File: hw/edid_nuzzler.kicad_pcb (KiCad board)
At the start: 2 copper layers, 49 x 32 mm, 49 parts, among them J1 HDMI_A, J2 HDMI_A, J4 USB_C_Receptacle_USB2.0_16P, J5 Prog, Q1 BSS84AK, SW1 SW_Push, U1 74LVC1G3157, U2 74LVC1G3157, U3 CH340N, U4 CH32V003AxMx, U5 74LVC1G3157, U6 ZD24C16A-STGMT

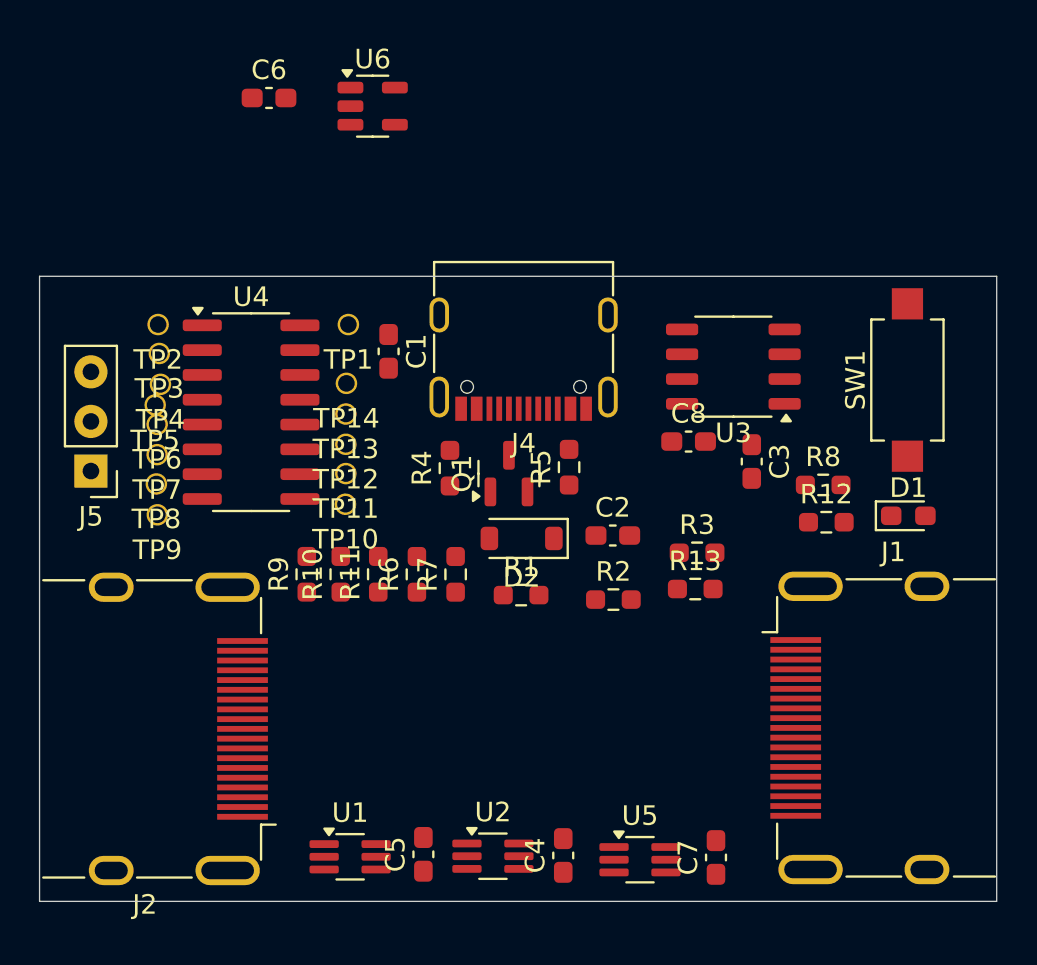
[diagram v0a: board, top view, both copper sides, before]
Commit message: Corase layout
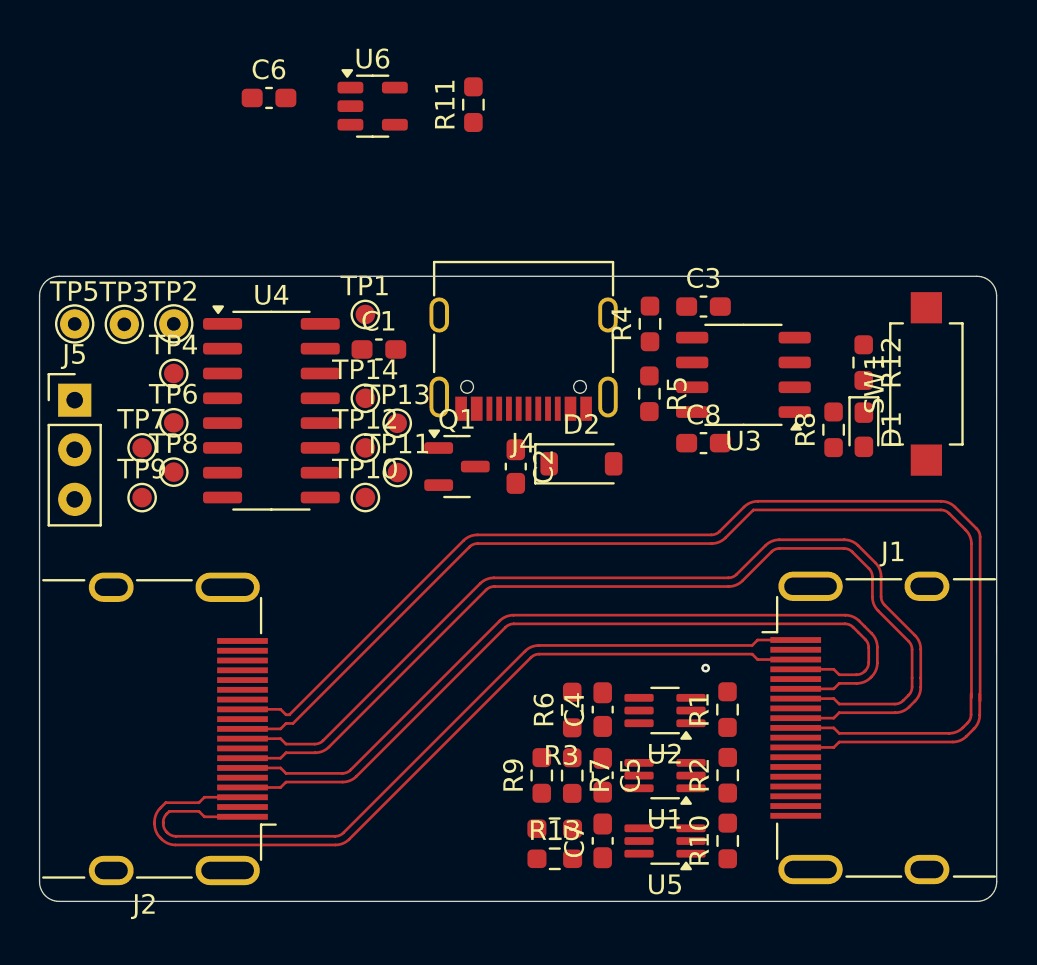
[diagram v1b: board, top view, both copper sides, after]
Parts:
- TP1, TP10, TP11, TP12, TP13, TP14, TP4, TP6, TP7, TP8, TP9: value ~ -> pad; footprint nuzzler:Pin_tight -> TestPoint:TestPoint_Pad_D1.0mm
- TP2, TP3, TP5: footprint nuzzler:Pin_tight -> TestPoint:TestPoint_THTPad_D1.5mm_Drill0.7mm
- moved R11 24.5 mm to (183.6, 53.3)
- moved R10 24.1 mm to (196.6, 91.0)
- moved U1 16.6 mm to (193.4, 87.7), turned to 180 degrees
- moved R3 15.9 mm to (187.8, 90.4)
- moved R9 15.8 mm to (187.1, 87.7)
- moved R13 15.6 mm to (187.8, 91.9)
- moved R4 12.6 mm to (192.7, 64.5)
- moved R1 12.1 mm to (196.6, 84.3), turned to 90 degrees
- moved R7 11.9 mm to (188.7, 87.7), turned to -90 degrees
- moved U2 11.5 mm to (193.4, 84.3), turned to 180 degrees
- moved R2 10.7 mm to (196.6, 87.6), turned to 90 degrees
- moved R6 10.6 mm to (188.7, 84.3)
- moved C5 10.0 mm to (190.2, 87.6), turned to -90 degrees
- moved R12 8.39 mm to (203.6, 66.5), turned to -90 degrees
- moved C3 8.31 mm to (195.4, 63.6), turned to 0 degrees
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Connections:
- net Net-(J1-CK+) renamed /CK+
- net Net-(J1-CK-) renamed /CK-
- net Net-(J1-D0+) renamed /D0+
- net Net-(J1-D0-) renamed /D0-
- net Net-(J1-D1+) renamed /D1+
- net Net-(J1-D1-) renamed /D1-
- net Net-(J1-D2+) renamed /D2+
- net Net-(J1-D2-) renamed /D2-
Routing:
- net /CK-: track 0.00 -> 62.8 mm
- net /CK+: track 0.00 -> 61.2 mm
- net /D0-: track 0.00 -> 51.6 mm
- net /D0+: track 0.00 -> 50.2 mm
- net /D2-: track 0.00 -> 42.8 mm
- net /D1-: track 0.00 -> 42.4 mm
- net /D2+: track 0.00 -> 41.4 mm
- net /D1+: track 0.00 -> 41.0 mm
- net GND: vias 0 -> 1
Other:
- outline, holes or cut-outs redrawn
- copper layers 2 -> 4

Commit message: Hopefully better high speed layout
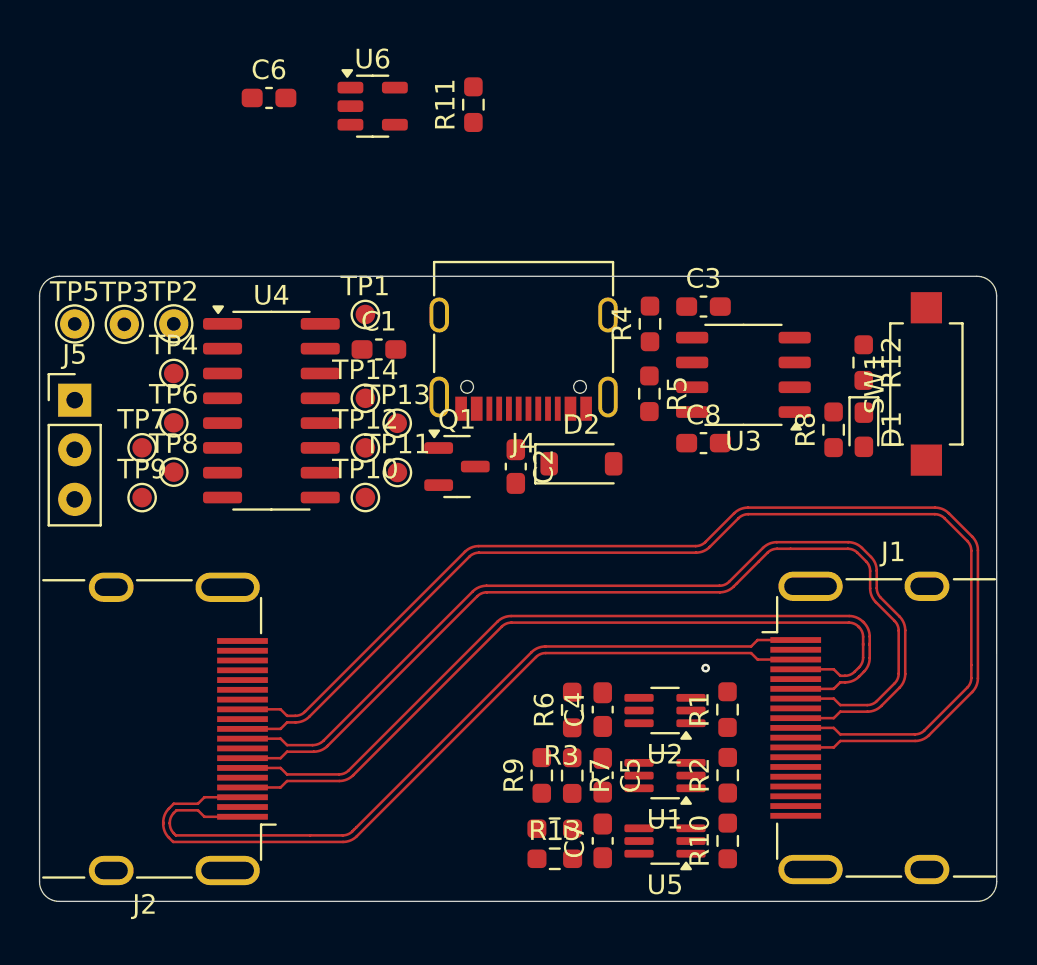
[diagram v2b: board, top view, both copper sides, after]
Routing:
- net /CK-: track 62.8 -> 60.6 mm
- net /CK+: track 61.2 -> 59.5 mm
- net /D0-: track 51.6 -> 50.0 mm
- net /D0+: track 50.2 -> 48.9 mm
- net /D2-: track 42.8 -> 41.9 mm
- net /D2+: track 41.4 -> 40.8 mm
- net /D1-: track 42.4 -> 41.9 mm

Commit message: PCB wip
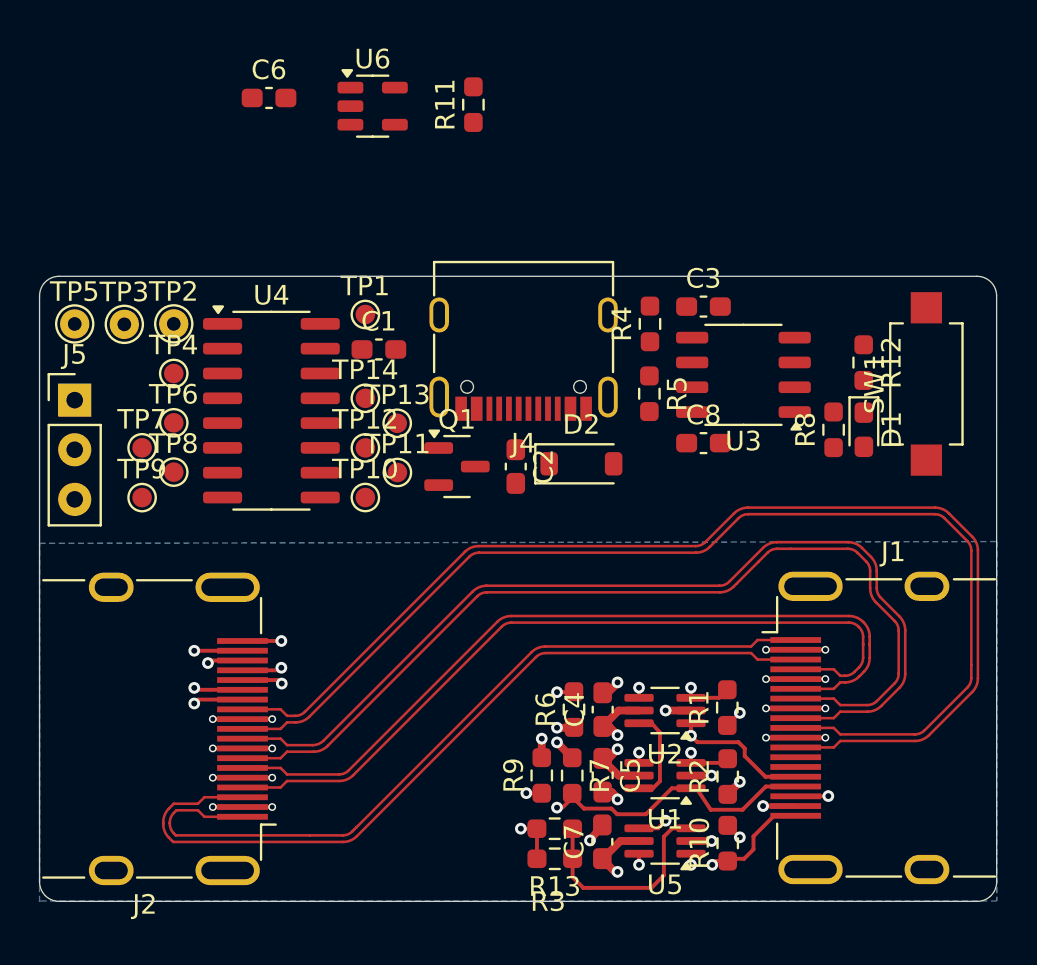
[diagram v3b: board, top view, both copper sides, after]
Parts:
- moved R10 0.12 mm to (196.6, 91.1)
- moved R1 0.10 mm to (196.6, 84.2)
- moved R6 0.09 mm to (188.8, 84.3)
- moved R2 0.07 mm to (196.6, 87.7)
- moved C7 0.05 mm to (190.2, 91.0)
- turned R13 to 180 degrees
- turned R3 to 180 degrees
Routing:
- net GND: track 0.00 -> 34.3 mm, vias 1 -> 24
- net Net-(J2-SDA): track 0.00 -> 28.5 mm, vias 0 -> 2
- net Net-(J2-SCL): track 0.00 -> 23.3 mm, vias 0 -> 2
- net +5V: track 0.00 -> 18.4 mm, vias 0 -> 10
- net Net-(J1-SDA): track 0.00 -> 14.6 mm, vias 0 -> 1
- net Net-(R13-Pad1): track 0.00 -> 11.2 mm
- net Net-(J1-SCL): track 0.00 -> 7.89 mm, vias 0 -> 2
- net Net-(J1-HPD): track 0.00 -> 7.18 mm, vias 0 -> 2
- net Net-(U4-PD4): track 0.00 -> 5.00 mm
- net Net-(J1-CEC): track 0.00 -> 2.55 mm, vias 0 -> 1
- net Net-(J5-Pin_3): track 0.00 -> 2.55 mm, vias 0 -> 1
- net Net-(J1-UTILITY): track 0.00 -> 2.52 mm, vias 0 -> 1
- net Net-(U4-PC6): track 0.00 -> 2.49 mm, vias 0 -> 1
- net Net-(J2-HPD): track 0.00 -> 2.47 mm, vias 0 -> 2
- net Net-(U4-PD7): track 0.00 -> 2.36 mm, vias 0 -> 1
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- added copper zone on B.Cu, net +5V
- added copper zone on In1.Cu, net GND

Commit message: Rough idea about routing
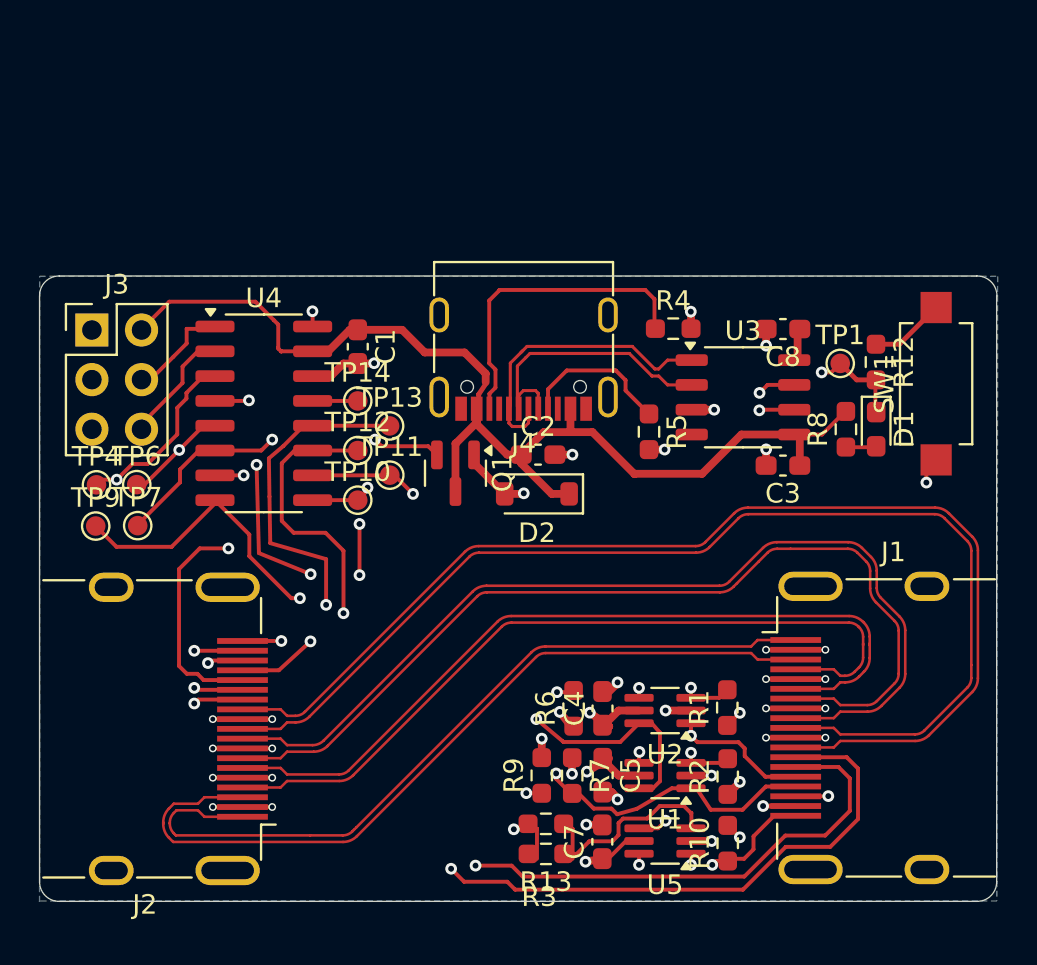
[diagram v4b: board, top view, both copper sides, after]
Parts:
- removed C6: 1u, Capacitor_SMD:C_0603_1608Metric_Pad1.08x0.95mm_HandSolder
- removed J5: Prog, nuzzler:PinHeader_1x03_P2.54mm_Vertical_Tight
- removed R11: 5k1, Resistor_SMD:R_0603_1608Metric_Pad0.98x0.95mm_HandSolder
- removed TP2, TP3, TP5: ~, TestPoint:TestPoint_THTPad_D1.5mm_Drill0.7mm
- removed TP8: pad, TestPoint:TestPoint_Pad_D1.0mm
- removed U6: ZD24C16A-STGMT, Package_TO_SOT_SMD:SOT-23-5
- added J3: Conn_02x03_Counter_Clockwise, Connector_PinHeader_2.54mm:PinHeader_2x03_P2.54mm_Vertical, F.Cu at (164.1, 64.8)
- moved TP1 24.4 mm to (202.4, 66.6)
- moved C3 9.10 mm to (199.5, 71.8), turned to 180 degrees
- moved C8 7.12 mm to (199.5, 64.8), turned to 180 degrees
- moved TP4 6.94 mm to (164.3, 72.8)
- moved TP7 3.99 mm to (166.4, 74.9)
- moved TP6 3.69 mm to (166.4, 72.8)
- moved TP9 2.79 mm to (164.3, 74.9)
- moved D2 2.75 mm to (186.9, 73.2), turned to 180 degrees
- moved R5 1.95 mm to (192.6, 70.1)
- moved C2 1.29 mm to (186.9, 71.2), turned to 0 degrees
- moved R4 1.21 mm to (193.8, 64.8), turned to 0 degrees
- moved U3 1.15 mm to (197.4, 68.3), turned to 0 degrees
- moved C1 1.09 mm to (177.7, 65.7), turned to -90 degrees
- moved D1 0.63 mm to (204.2, 69.9)
- moved R12 0.63 mm to (204.2, 66.5)
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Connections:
- net Net-(U3-UD+) renamed /UD+
- net Net-(U3-UD-) renamed /UD-
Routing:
- net Net-(J1-SCL): track 7.89 -> 67.0 mm, vias 2 -> 4
- net Net-(D2-K): track 0.00 -> 57.4 mm
- net Net-(U4-PC3): track 0.54 -> 51.0 mm, vias 1 -> 2
- net Net-(J1-CEC): track 2.55 -> 48.5 mm, vias 1 -> 2
- net Net-(J1-HPD): track 7.18 -> 52.7 mm
- net Net-(J1-UTILITY): track 2.52 -> 46.2 mm, vias 1 -> 2
- net Net-(U4-PC4): track 0.89 -> 43.2 mm, vias 1 -> 2
- net Net-(J1-SDA): track 14.6 -> 55.1 mm, vias 1 -> 3
- net Net-(U4-PC6): track 2.49 -> 42.1 mm, vias 1 -> 2
- net Net-(J3-Pin_3): track 2.55 -> 42.1 mm, vias 1 -> 2
- net Net-(U4-PD4): track 5.00 -> 41.4 mm, vias 0 -> 2
- net Net-(U4-PA1): track 0.79 -> 34.8 mm, vias 1 -> 2
- net Net-(D1-K): track 0.00 -> 33.1 mm, vias 0 -> 2
- net Net-(U4-PD7): track 2.36 -> 33.4 mm, vias 1 -> 2
- net Net-(U3-RXD): track 0.00 -> 27.2 mm, vias 0 -> 2
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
